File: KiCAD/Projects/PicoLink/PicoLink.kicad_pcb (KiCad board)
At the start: 2 copper layers, 53.2 x 24.8 mm, 46 parts, among them J1 USB_C_Receptacle_GCT_USB4110-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, J5 Conn_01x03, J6 Conn_01x03, SW1 434123025826_BTN, U1 W25Q16JV, U3 SWD_JTAG_10pin, U5 AP2112K-3.3, Y1 CSTNE12M0GH5L000R0

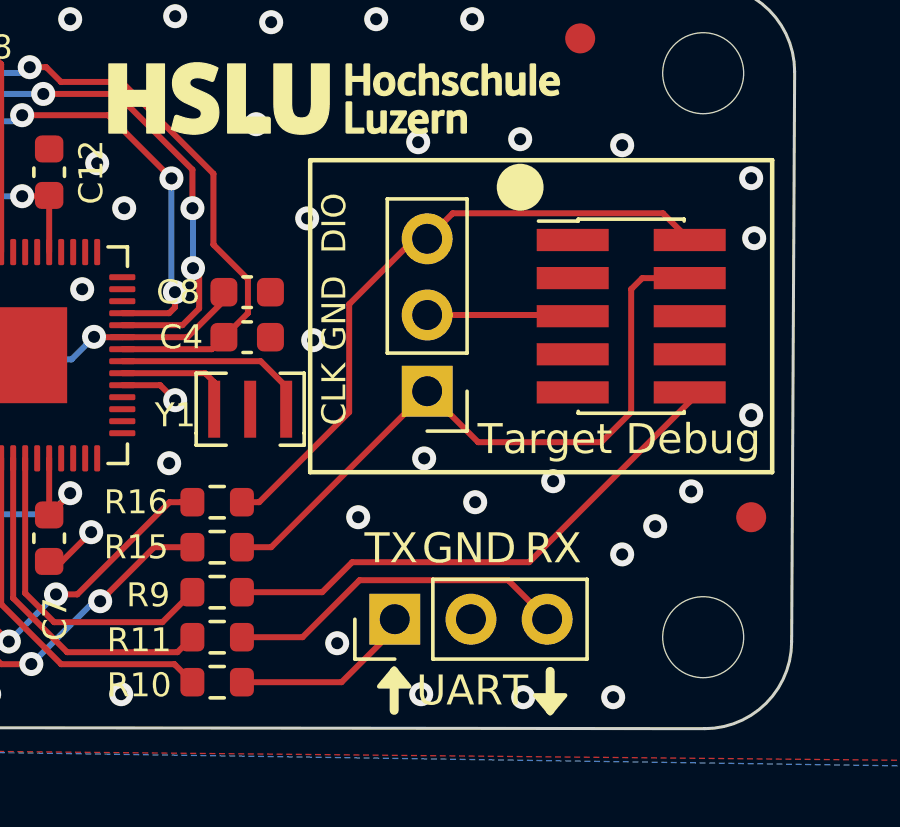
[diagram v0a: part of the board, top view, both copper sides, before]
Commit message: added open points
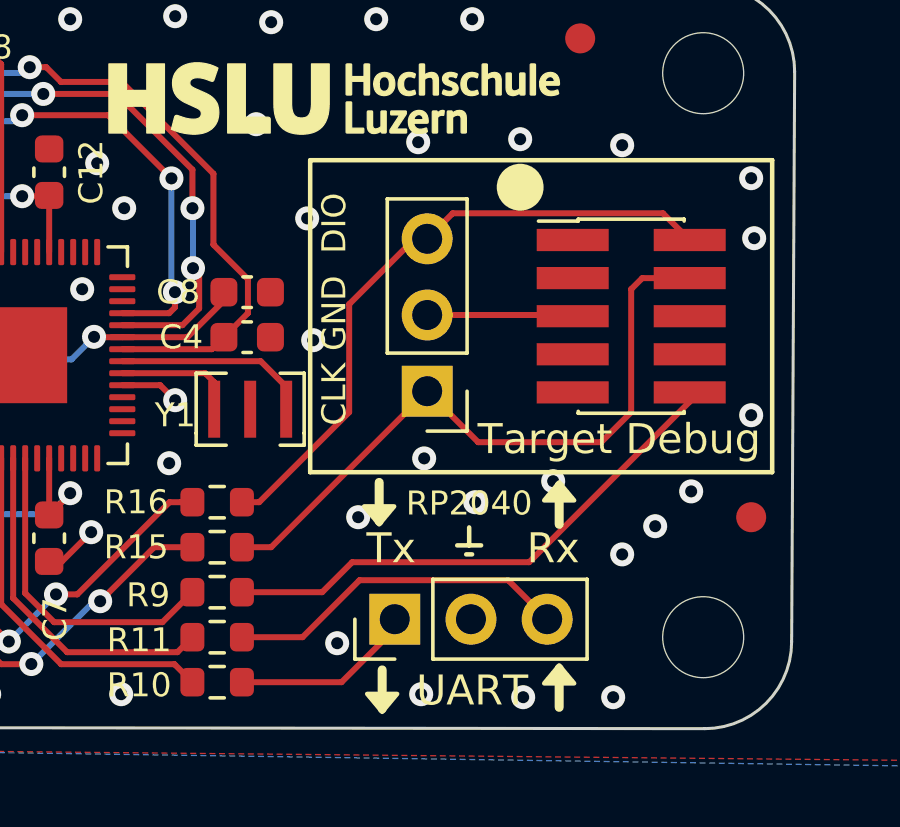
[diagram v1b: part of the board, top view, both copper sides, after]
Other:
- board text added: "RP2040"
- board text added: "Rx"
- board text added: "Tx"
- board text removed: "RX"
- board text removed: "TX"
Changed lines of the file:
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@@
       ) (layer "B.SilkS") (width 0.01) (fill solid))
   )
+  (gr_line (start 126 126.3) (end 126 127.6) (layer "F.SilkS") (width 0.3))
+  (gr_line (start 128.9 128.7) (end 129.1 128.7) (layer "F.SilkS") (width 0.15))
   (gr_rect (start 123.700156 115.560476) (end 139.100156 125.960476) (layer "F.SilkS") (width 0.15) (fill none))
   (gr_poly
     (pts
-      (xy 131.2 133.4)
-      (xy 132.2 133.4)
-      (xy 131.7 134)
+      (xy 125.5 127.1)
+      (xy 126.5 127.1)
+      (xy 126 127.7)
     ) (layer "F.SilkS") (width 0.15) (fill solid))
   (gr_poly
     (pts
-      (xy 127 133.1)
-      (xy 126 133.1)
-      (xy 126.5 132.5)
+      (xy 125.6 133.35)
+      (xy 126.6 133.35)
+      (xy 126.1 133.95)
     ) (layer "F.SilkS") (width 0.15) (fill solid))
-  (gr_line (start 126.5 133.9) (end 126.5 132.6) (layer "F.SilkS") (width 0.3))
-  (gr_line (start 131.7 132.6) (end 131.7 133.9) (layer "F.SilkS") (width 0.3))
+  (gr_poly
+    (pts
+      (xy 132.5 126.9)
+      (xy 131.5 126.9)
+      (xy 132 126.3)
+    ) (layer "F.SilkS") (width 0.15) (fill solid))
+  (gr_poly
+    (pts
+      (xy 132.5 133)
+      (xy 131.5 133)
+      (xy 132 132.4)
+    ) (layer "F.SilkS") (width 0.15) (fill solid))
+  (gr_line (start 132 133.8) (end 132 132.5) (layer "F.SilkS") (width 0.3))
+  (gr_line (start 126.1 132.55) (end 126.1 133.85) (layer "F.SilkS") (width 0.3))
+  (gr_line (start 128.6 128.4) (end 129.4 128.4) (layer "F.SilkS") (width 0.15))
+  (gr_line (start 129 128.4) (end 129 127.8) (layer "F.SilkS") (width 0.15))
+  (gr_line (start 132 127.7) (end 132 126.4) (layer "F.SilkS") (width 0.3))
   (gr_line (start 86.65061 112.6) (end 86.65061 131.549387) (layer "Edge.Cuts") (width 0.1))
   (gr_arc (start 89.55061 134.449387) (mid 87.499997 133.6) (end 86.65061 131.549387) (layer "Edge.Cuts") (width 0.1))
@@
   )
   (gr_text "CLK" (at 124.5 123.360476 90) (layer "F.SilkS")
-    (effects (font (size 0.8 0.8) (thickness 0.1)))
+    (effects (font (size 0.8 0.8) (thickness 0.2)))
   )
   (gr_text "Boot Sel" (at 98.7 132.3) (layer "F.SilkS")
     (effects (font (size 1 1) (thickness 0.15)))
   )
-  (gr_text "TX" (at 126.4 128.5) (layer "F.SilkS")
+  (gr_text "Tx" (at 126.4 128.5) (layer "F.SilkS")
     (effects (font (size 1 1) (thickness 0.15)))
   )
-  (gr_text "DIO" (at 124.5 117.660476 90) (layer "F.SilkS")
+  (gr_text "RP2040" (at 129 127) (layer "F.SilkS")
     (effects (font (size 0.8 0.8) (thickness 0.1)))
   )
+  (gr_text "DIO" (at 124.5 117.660476 90) (layer "F.SilkS")
+    (effects (font (size 0.8 0.8) (thickness 0.2)))
+  )
   (gr_text "GND" (at 124.5 120.660476 90) (layer "F.SilkS")
-    (effects (font (size 0.8 0.8) (thickness 0.1)))
+    (effects (font (size 0.8 0.8) (thickness 0.2)))
   )
-  (gr_text "GND" (at 129 128.5) (layer "F.SilkS")
+  (gr_text "Rx" (at 131.8 128.5) (layer "F.SilkS")
     (effects (font (size 1 1) (thickness 0.15)))
   )
-  (gr_text "RX" (at 131.8 128.5) (layer "F.SilkS")
-    (effects (font (size 1 1) (thickness 0.15)))
-  )
